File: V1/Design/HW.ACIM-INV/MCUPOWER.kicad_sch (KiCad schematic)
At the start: 9 parts, among them J14 MCU PWR, J15 INV PWR & RELAYS, U6 LDO 3.3V±0.1%/20mA

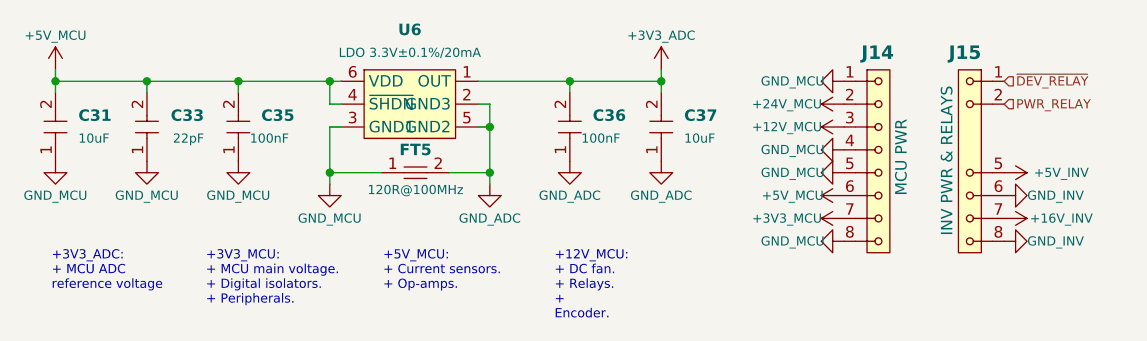
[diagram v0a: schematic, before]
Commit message: V1 schematic update 22
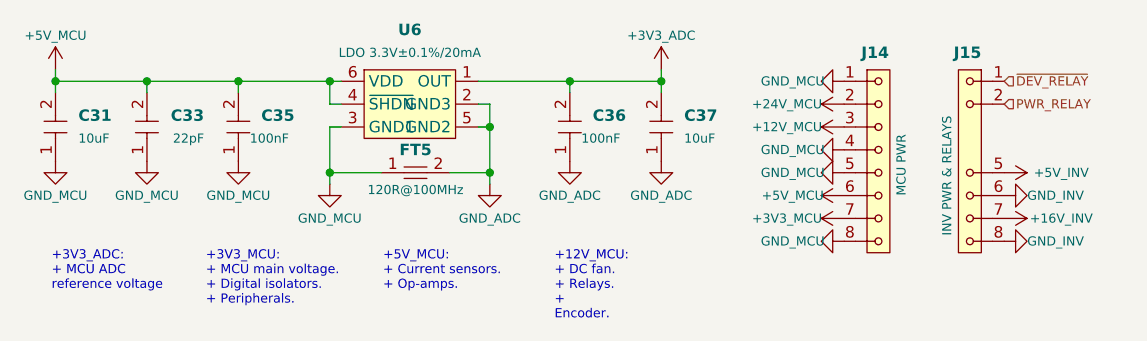
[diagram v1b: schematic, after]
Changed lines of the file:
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@@
 			(effects
 				(font
-					(size 1.5 1.5)
+					(face "Consolas")
+					(size 1.27 1.27)
 					(bold yes)
 				)
@@
 			(effects
 				(font
-					(size 1.27 1.27)
+					(face "Consolas")
+					(size 1.016 1.016)
+					(thickness 0.254)
 				)
 				(justify left)
@@
 			(effects
 				(font
-					(size 1.27 1.27)
+					(face "Consolas")
+					(size 1.016 1.016)
+					(thickness 0.254)
 				)
 				(hide yes)
@@
 			(effects
 				(font
-					(size 1.27 1.27)
+					(face "Consolas")
+					(size 1.016 1.016)
+					(thickness 0.254)
 				)
 				(hide yes)
@@
 			(effects
 				(font
-					(size 1.27 1.27)
+					(face "Consolas")
+					(size 1.016 1.016)
+					(thickness 0.254)
 				)
 				(hide yes)
@@
 			(effects
 				(font
-					(size 1.27 1.27)
+					(face "Consolas")
+					(size 1.016 1.016)
+					(thickness 0.254)
 				)
 				(hide yes)
@@
 			(effects
 				(font
-					(size 1.27 1.27)
+					(face "Consolas")
+					(size 1.016 1.016)
+					(thickness 0.254)
 				)
 				(hide yes)
@@
 			(effects
 				(font
-					(size 1.27 1.27)
+					(face "Consolas")
+					(size 1.016 1.016)
+					(thickness 0.254)
 				)
 				(hide yes)
@@
 			(effects
 				(font
-					(size 1.27 1.27)
+					(face "Consolas")
+					(size 1.016 1.016)
+					(thickness 0.254)
 				)
 				(hide yes)
@@
 			(effects
 				(font
-					(size 1.5 1.5)
+					(face "Consolas")
+					(size 1.27 1.27)
 					(bold yes)
 				)
@@
 			(effects
 				(font
-					(size 1.27 1.27)
+					(face "Consolas")
+					(size 1.016 1.016)
+					(thickness 0.254)
 				)
 				(justify left)
@@
 			(effects
 				(font
-					(size 1.27 1.27)
+					(face "Consolas")
+					(size 1.016 1.016)
+					(thickness 0.254)
 				)
 				(hide yes)
@@
 			(effects
 				(font
-					(size 1.27 1.27)
+					(face "Consolas")
+					(size 1.016 1.016)
+					(thickness 0.254)
 				)
 				(hide yes)
@@
 			(effects
 				(font
-					(size 1.27 1.27)
+					(face "Consolas")
+					(size 1.016 1.016)
+					(thickness 0.254)
 				)
 				(hide yes)
@@
 			(effects
 				(font
-					(size 1.27 1.27)
+					(face "Consolas")
+					(size 1.016 1.016)
+					(thickness 0.254)
 				)
 				(hide yes)
@@
 			(effects
 				(font
-					(size 1.27 1.27)
+					(face "Consolas")
+					(size 1.016 1.016)
+					(thickness 0.254)
 				)
 				(hide yes)
@@
 			(effects
 				(font
-					(size 1.27 1.27)
+					(face "Consolas")
+					(size 1.016 1.016)
+					(thickness 0.254)
 				)
 				(hide yes)
@@
 			(effects
 				(font
-					(size 1.27 1.27)
-				)
-				(hide yes)
+					(face "Consolas")
+					(size 1.016 1.016)
+					(thickness 0.254)
+				)
+				(hide yes)
